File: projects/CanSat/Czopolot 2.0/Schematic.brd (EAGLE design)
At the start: 53 x 31.8 mm, 88 parts, among them X1 FH12-24S-0.5SH

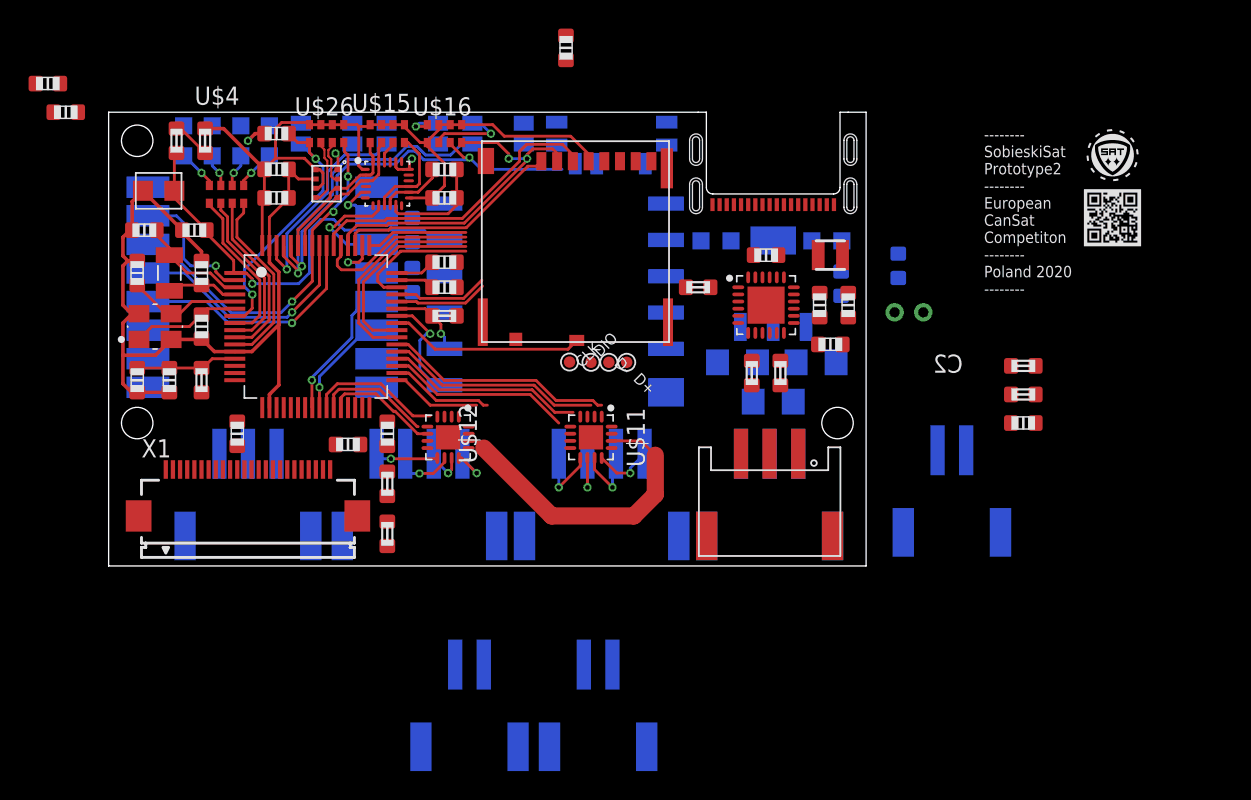
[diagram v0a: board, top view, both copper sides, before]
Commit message: V2 work...
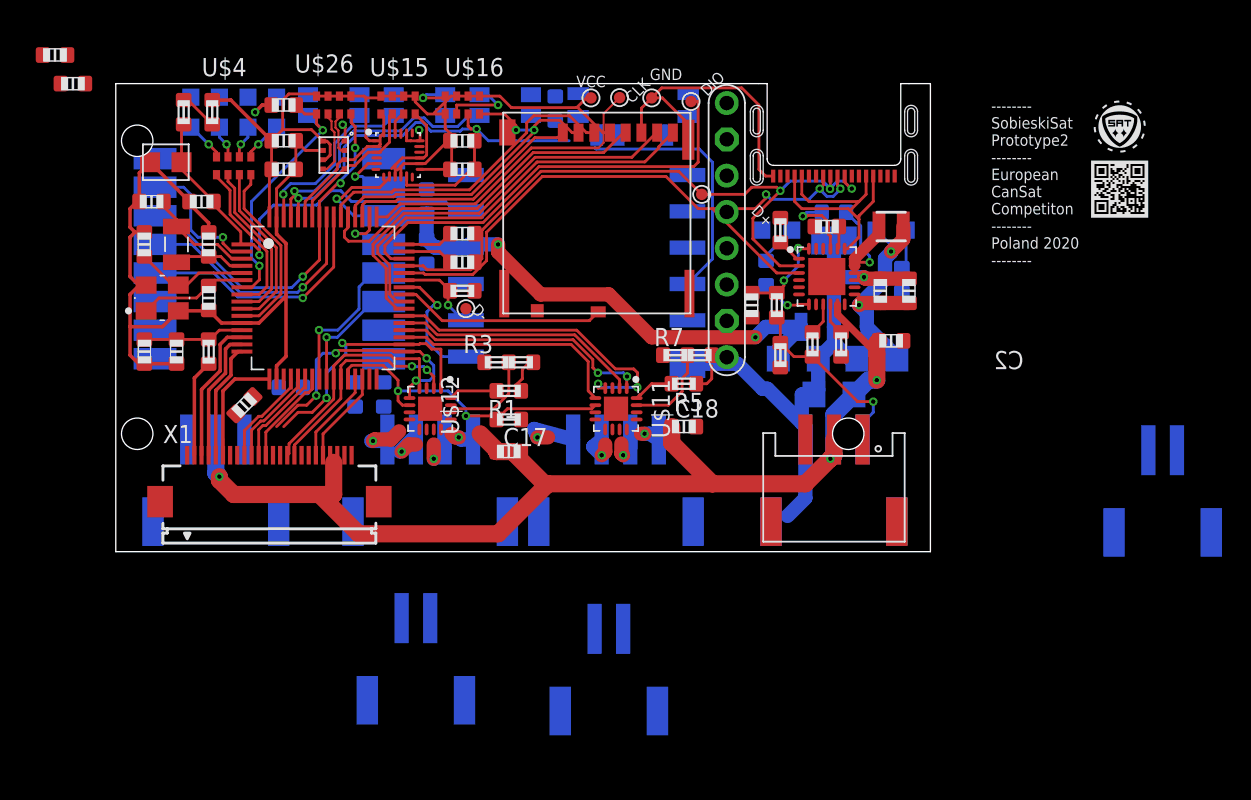
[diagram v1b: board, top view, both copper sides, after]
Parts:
- removed THR: NTC, SobieskiSat2:NTC
- added C17, C18: 100n, Unified:C0603
- added GND, VCC: PADTEST, Unified:TESTPAD
- added R1, R5: 10k, Unified:R0603
- added R3, R7: 10k, SobieskiSat2:DR0603
- added R8: 1k, Unified:R0603
- added U$25: GPIO_PADS, SobieskiSat2:GPIO_PADS
- moved C20 20.7 mm to (44.5, 17.2), turned to 90 degrees
- moved DIO 19.5 mm to (40.2, 31.5)
- moved CLK 18.8 mm to (35.2, 31.8)
- moved R22 17.8 mm to (46.2, 17.2), turned to 90 degrees
- moved R23 17.2 mm to (46.5, 13.8), turned to 90 degrees
- moved BAT_PACK 14.8 mm to (73.2, 3.75)
- moved D+ 12.9 mm to (41.0, 25.0)
- moved R2 11.7 mm to (27.5, 9.25), turned to 180 degrees
- moved D- 10.7 mm to (24.5, 17.0)
- moved R4 9.55 mm to (12.2, 11.5), flipped to the bottom, turned to 0 degrees
- moved R20 7.00 mm to (46.5, 22.5), turned to 270 degrees
- moved C21 5.86 mm to (50.2, 23.8), turned to 0 degrees
- moved U$13 4.96 mm to (21.0, -8.00)
- moved C22 4.70 mm to (49.8, 22.8)
- moved L2 4.70 mm to (54.2, 22.8)
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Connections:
- removed net GPS_RST: U$3.10
- removed net N$22: R22.1, R23.2, R24.1, THR.P$1
- removed net N$25: R0.1
- new net N$36: R1.2, U$12.16
- new net N$39: R3.1, U$12.15
- new net N$40: R5.2, U$11.16
- new net N$42: R7.1, U$11.15
- new net NTC: R22.1, R23.2, R24.1, U$24.P$3
- new net UART2_RX: U$1.17, X1.6
- new net UART2_TX: U$1.16, X1.5
- new net UART4_RX: U$1.15, X1.4
- new net UART4_TX: U$1.14, X1.3
- net BAT: now also C17.1, C18.1, U$19.P$2, U$20.P$2, U$24.P$2, X1.21, X1.22
- net DFU: now also U$3.10
- net EN_1: now also U$12.5, X1.13
- net EN_2: now also U$12.1, X1.14
- net GND: now also C17.2, C18.2, GND.PAD, R0.1, R3.3, R7.3, U$19.P$1, U$20.P$1, U$24.P$1, X1.1, X1.17, X1.23, X1.7; no longer THR.P$2
- net GPIO_DAC: now also X1.9
- net GPIO_MISO: now also X1.11
- net GPIO_MOSI: now also X1.12
- net GPIO_SCK: now also X1.10
- net GPIO_SCL: now also X1.20
- net GPIO_SDA: now also X1.19
- net N$10: now also R8.1
- net N$3: now also R8.2
- net PWM_1: now also U$12.2, X1.16
- net PWM_2: now also U$12.4, X1.15
- net PWM_3: now also U$11.2
- net PWM_4: now also U$11.4
- net P_EN_3: now also U$11.5
- net P_EN_4: now also U$11.1
- net VCC: now also R1.1, R3.2, R5.1, R7.2, VCC.PAD, X1.18, X1.2, X1.24, X1.8
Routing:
- net GND: track 75.8 -> 136.0 mm, vias 4 -> 5
- net BAT: track 22.1 -> 79.9 mm, vias 0 -> 3
- net VCC: track 64.6 -> 118.3 mm, vias 1 -> 3
- net USB_D+: track 6.59 -> 47.6 mm, vias 0 -> 3
- net USB_D-: track 6.53 -> 46.9 mm, vias 0 -> 3
- net SWDIO: track 8.85 -> 31.1 mm
- net USB_VBUS: track 0.00 -> 21.2 mm
- net VSYS: track 0.00 -> 17.2 mm, vias 0 -> 2
- net SD_D1: track 13.5 -> 28.9 mm
- net DFU: track 28.1 -> 43.4 mm
- net SWCLK: track 7.13 -> 21.7 mm
- net MOT_STBY: track 8.02 -> 22.5 mm, vias 0 -> 2
- net SD_D0: track 14.7 -> 28.8 mm
- net NTC: track 0.00 -> 13.1 mm, vias 0 -> 1
- net SD_CLK: track 11.6 -> 24.5 mm
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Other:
- board size 53 x 31.8 mm -> 57 x 32.8 mm

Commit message: V2 almost done
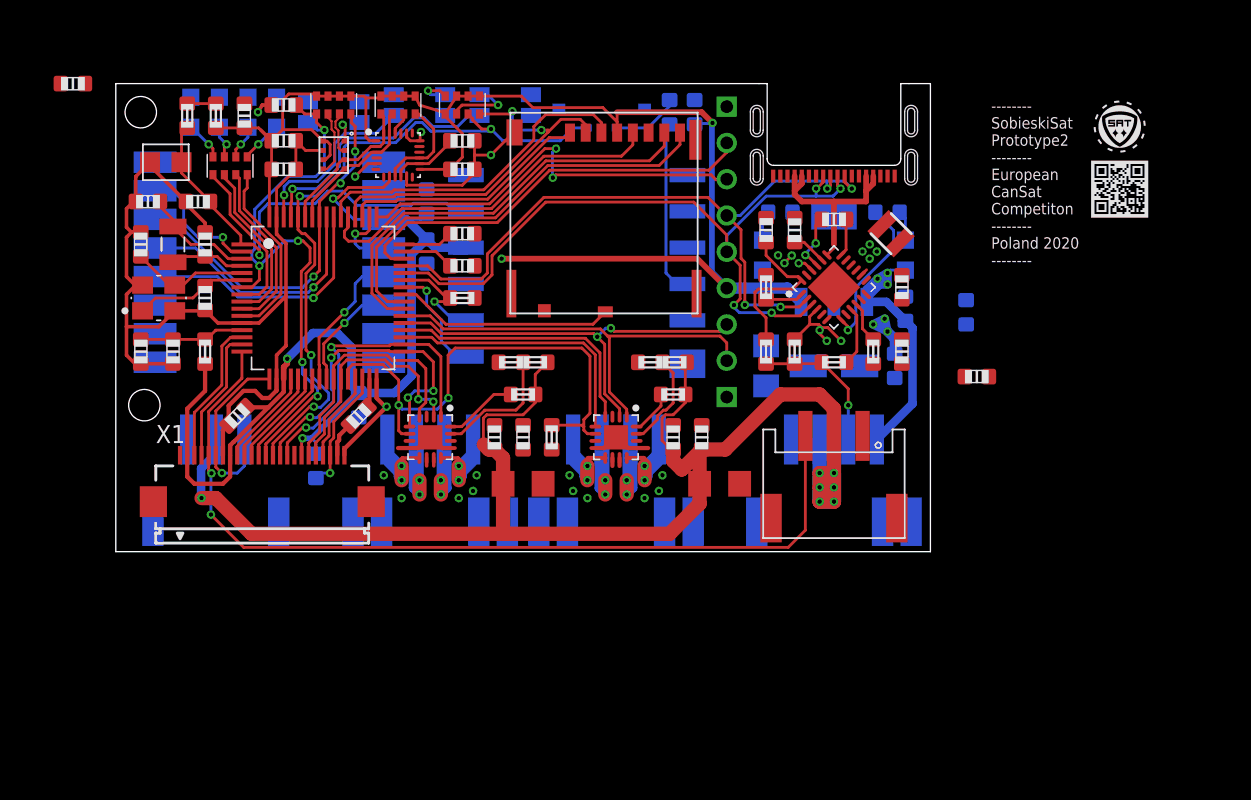
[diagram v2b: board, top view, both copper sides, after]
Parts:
- removed BAT_PACK: (no value), SobieskiSat2:2X_JSTSMD_F
- removed CLK, D+, D-, DIO, GND, VCC: PADTEST, Unified:TESTPAD
- removed U$18: CONNECTOR_F_X4_JST_SMD, Unified:4X_JSTSMD_F
- removed U$24: CONNECTOR_F_X3_JST_SMD, Unified:3X_JSTSMD_F
- added C19, C25: 10u, Unified:C1206
- added C26, C27: 50p, Unified:C0603
- added C28: (no value), rcl:153CLV-0405
- added R10, R9: 0R, Unified:R0603
- C2, C23: device Unified:C1206 -> Unified:C0603
- U$13: value MOTORJST_SMD -> MOTOR_DUO; device Unified:2X_JSTSMD_F -> SobieskiSat2:4(2)X_JSTSMD_F
- U$14: value MOTORJST_SMD -> BAT_JST_4(3); device Unified:2X_JSTSMD_F -> SobieskiSat2:4(3)X_JSTSMD_F
- U$17: value CONNECTOR_F_X4_JST_SMD -> MOTOR_DUO; device Unified:4X_JSTSMD_F -> SobieskiSat2:4(2)X_JSTSMD_F
- U$25: value GPIO_PADS -> GPIO_DEBUG; device SobieskiSat2:GPIO_PADS -> SobieskiSat2:GPIO_DEBUG
- X1: device con-hirose:FH12-24S-0.5SH -> SobieskiSat2:FH12-24S-0.5SH
- moved U$14 20.6 mm to (50.2, 4.50)
- moved U$13 18.8 mm to (35.0, 4.50)
- moved C80 13.9 mm to (9.00, 30.5), turned to 90 degrees
- moved C16 9.75 mm to (40.5, 30.8), turned to 270 degrees
- moved R30 9.74 mm to (46.5, 23.8), turned to 180 degrees
- moved R8 9.50 mm to (54.0, 23.8), turned to 180 degrees
- moved LEDCH 9.17 mm to (55.2, 20.8), turned to 0 degrees
- moved LEDP 9.17 mm to (45.2, 20.8), turned to 0 degrees
- moved C2 7.04 mm to (59.5, 16.8), turned to 270 degrees
- moved C10 6.50 mm to (60.2, 12.2)
- moved R4 5.77 mm to (14.0, 6.00), turned to 270 degrees
- moved C23 5.62 mm to (55.0, 14.0), flipped to the top, turned to 270 degrees
- moved C20 5.34 mm to (45.5, 22.5), turned to 270 degrees
- moved R20 4.12 mm to (45.5, 18.5)
- moved R22 3.34 mm to (45.5, 14.0)
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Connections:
- new net BAT_BQ: C23.1, R9.2, U$10.11, U$10.12
- new net GPS_RST: R10.2, U$3.10
- new net N$25: BTN_DFU.P$1, R10.1
- net BAT: now also C19.1, C25.1, C26.1, C27.1, R1.1, R3.2, R5.1, R7.2, R9.1, U$14.BAT; no longer BAT_PACK.+, C23.1, U$10.11, U$10.12, U$24.P$2, X1.21, X1.22
- net DFU: now also BTN_DFU.P$3, X1.14; no longer U$3.10
- net EN_1: now also X1.15; no longer X1.13
- net EN_2: now also X1.16; no longer X1.14
- net GND: now also BTN_DFU.P$2, C19.2, C25.2, C26.2, C27.2, U$13.S$1, U$13.S$2, U$13.S$3, U$13.S$4, U$14.GND, U$14.S$1, U$14.S$2, U$14.S$3, U$17.S$1, U$17.S$2, U$17.S$3, U$17.S$4, U$19.S$1, U$19.S$2, U$20.S$1, U$20.S$2, U$25.P$1, U$25.P$9, X1.S$1, X1.S$2; no longer BAT_PACK.-, GND.PAD, U$24.P$1
- net GPIO_SCL: now also X1.22; no longer X1.20
- net GPIO_SDA: now also X1.21; no longer X1.19
- net N$23: now also U$13.P$2; no longer U$18.P$2
- net N$29: now also U$13.P$3; no longer U$18.P$3
- net N$30: now also U$13.P$4; no longer U$18.P$4
- net N$4: now also U$13.P$1; no longer U$18.P$1
- net NRST: now also X1.13
- net NTC: now also U$14.NTC; no longer U$24.P$3
- net PWM_1: now also X1.20; no longer X1.16
- net PWM_2: now also X1.19; no longer X1.15
- net PWM_3: now also U$25.P$7
- net PWM_4: now also U$11.1, U$25.P$8; no longer U$11.4
- net P_EN_4: now also U$11.4; no longer U$11.1
- net SWCLK: now also U$25.P$3; no longer CLK.PAD
- net SWDIO: now also U$25.P$2; no longer DIO.PAD
- net UART2_RX: now also U$20.P$3
- net UART2_TX: now also U$19.P$3
- net USB_D+: now also U$25.P$4; no longer D+.PAD
- net USB_D-: now also U$25.P$5; no longer D-.PAD
- net VCC: now also LEDP.A, U$25.P$6; no longer LEDCH.A, R1.1, R3.2, R5.1, R7.2, VCC.PAD
- net VSYS: now also LEDCH.A, U$14.AUX; no longer LEDP.A
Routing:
- net VCC: track 118.3 -> 182.7 mm, vias 3 -> 6
- net UART2_TX: track 8.17 -> 62.1 mm, vias 0 -> 2
- net GND: track 136.0 -> 105.5 mm, vias 5 -> 19
- net BAT: track 79.9 -> 105.8 mm, vias 3 -> 7
- net NRST: track 18.7 -> 41.2 mm, vias 2 -> 5
- net MOT_STBY: track 22.5 -> 35.2 mm
- net PWM_3: track 17.3 -> 29.8 mm, vias 0 -> 2
- net GPS_RST: track 0.00 -> 12.3 mm
- net PWM_4: track 22.7 -> 30.8 mm, vias 2 -> 0
- net SWCLK: track 21.7 -> 29.1 mm, vias 0 -> 2
- net N$10: track 3.71 -> 11.0 mm
- net N$29: track 2.17 -> 8.89 mm, vias 1 -> 2
- net USB_VBUS: track 21.2 -> 14.7 mm
- net N$21: track 8.84 -> 2.64 mm, vias 1 -> 0
- net N$30: track 1.36 -> 7.55 mm, vias 1 -> 2
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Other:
- board text removed: "A"
- board text removed: "B"
- board text removed: "C"
- board text removed: "CH"
- board text removed: "D"
- board text removed: "DFU"
- board text removed: "PWR"
- board text removed: "USR"

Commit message: GND yet to fix
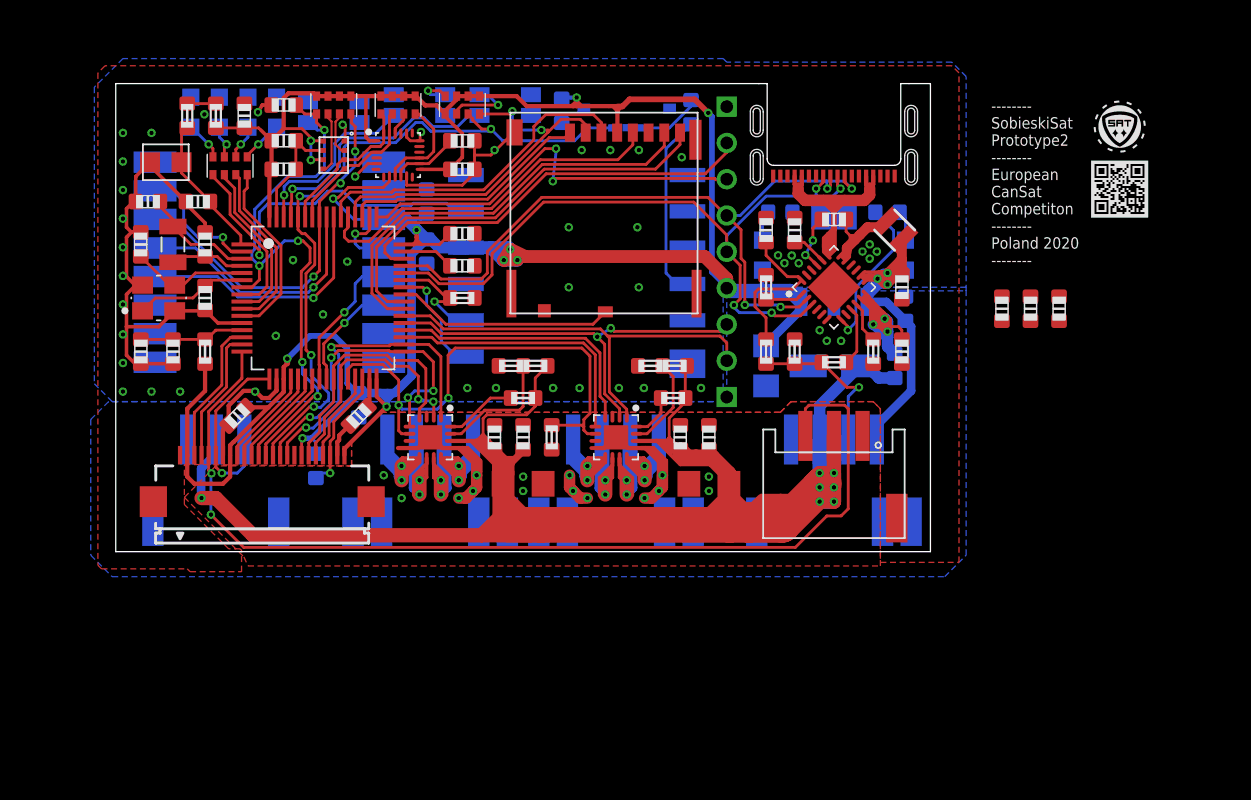
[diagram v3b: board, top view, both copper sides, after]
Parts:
- moved C81 68.8 mm to (64.0, 17.0), turned to 270 degrees
- moved C16 9.30 mm to (31.2, 30.9), turned to 90 degrees
- moved C10 7.46 mm to (66.0, 17.0), turned to 270 degrees
- moved C2 2.51 mm to (62.0, 17.0), flipped to the top
- moved BTN_DFU 1.75 mm to (35.8, 31.0)
- moved R10 1.50 mm to (40.2, 30.8)
- moved C25 0.75 mm to (41.5, 4.75), turned to 180 degrees
- moved C18 0.50 mm to (41.5, 8.00)
- moved C26 0.50 mm to (39.5, 8.00)
- moved L2 0.35 mm to (54.5, 22.5)
- moved R1 0.25 mm to (28.5, 10.8)
- moved R3 0.25 mm to (28.5, 13.0)
- moved R5 0.25 mm to (39.0, 10.8)
- moved R7 0.25 mm to (38.2, 13.0)
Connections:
- net BAT: now also C28.+, U$19.S$1, U$19.S$2
- net GND: now also C28.-; no longer U$19.S$1, U$19.S$2
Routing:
- net BAT: track 105.8 -> 157.2 mm
- net VCC: track 182.7 -> 204.3 mm, vias 6 -> 12
- net VSYS: track 21.0 -> 33.5 mm
- net BAT_BQ: track 4.69 -> 17.0 mm
- net UART2_TX: track 62.1 -> 71.2 mm
- net N$21: track 2.64 -> 9.75 mm
- net N$29: track 8.89 -> 15.2 mm
- net N$23: track 8.29 -> 14.2 mm
- net N$34: track 8.29 -> 13.8 mm
- net N$33: track 8.49 -> 13.7 mm
- net USB_VBUS: track 14.7 -> 19.8 mm
- net N$30: track 7.55 -> 11.8 mm
- net N$35: track 7.55 -> 11.5 mm
- net N$31: track 7.56 -> 10.5 mm
- net N$4: track 7.55 -> 10.5 mm
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- added copper zone on layer 1, net GND
- added copper zone on layer 16, net GND
